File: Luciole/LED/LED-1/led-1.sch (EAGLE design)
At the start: 6 parts, among them Q2 MOSFET-NCHANNELAO3404A

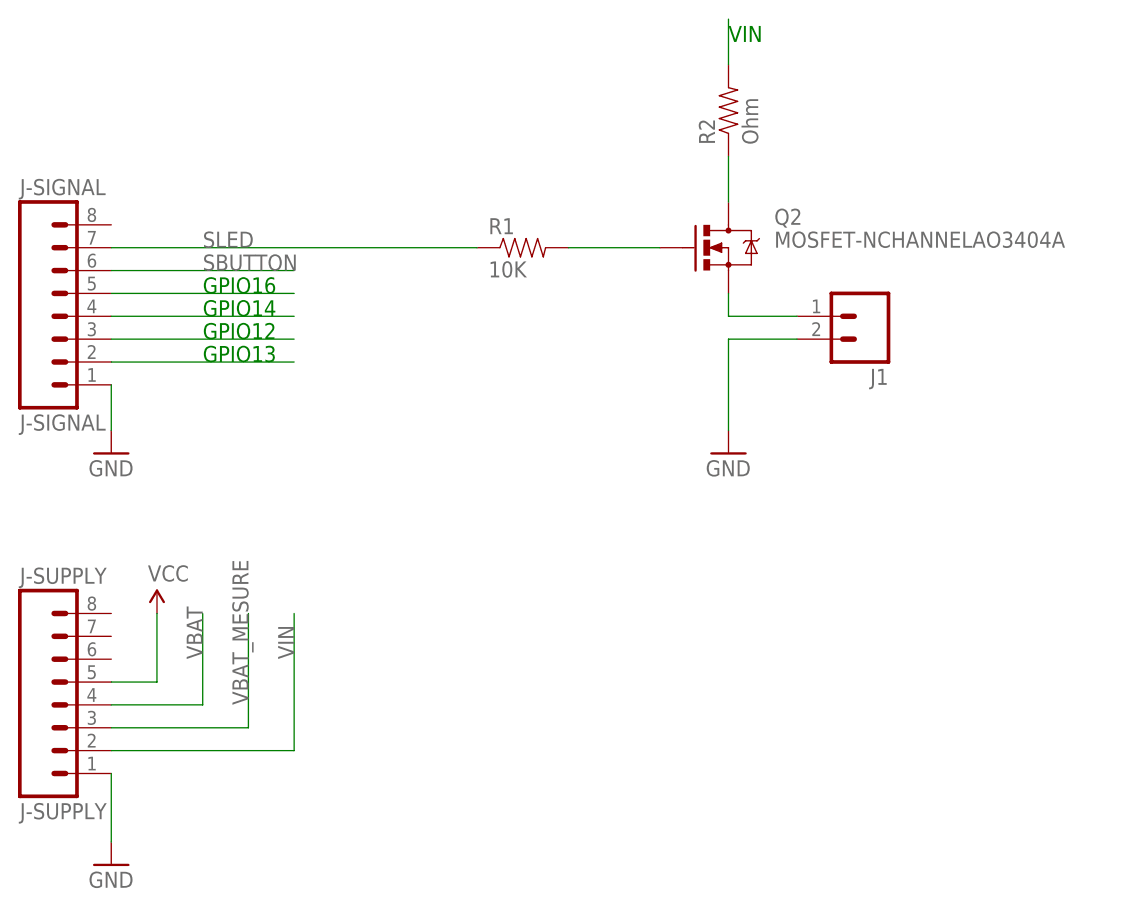
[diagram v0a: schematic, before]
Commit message: V2 de la Baballe
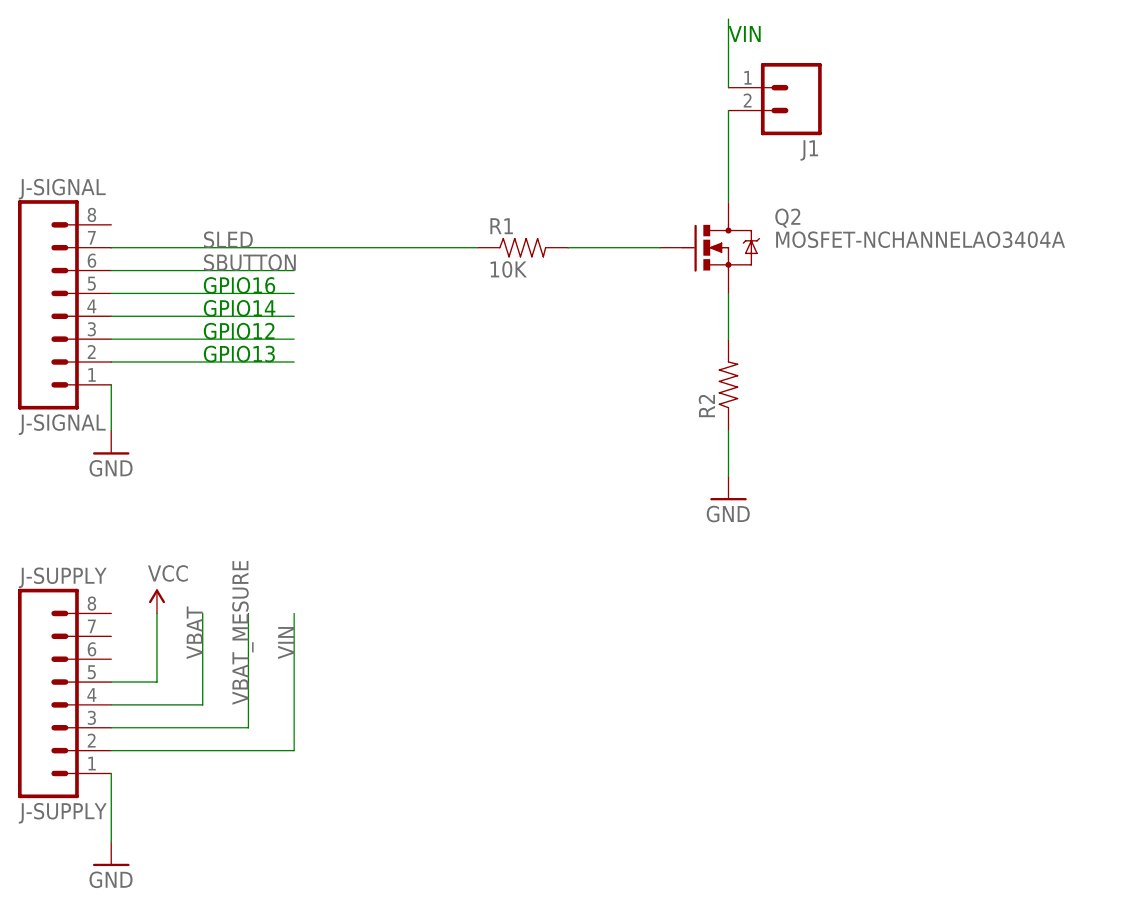
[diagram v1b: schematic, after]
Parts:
- R2: value Ohm -> (none); device SparkFun-Passives:RESISTORPTH-1/4W -> SparkFun-Passives:RESISTORPTH-1/2W
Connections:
- net GND: now also R2.1; no longer J1.2
- net N$1: now also R2.2; no longer J1.1
- net N$3: now also J1.2; no longer R2.1
- net VIN: now also J1.1; no longer R2.2
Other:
- moved on the sheet: J1, R2
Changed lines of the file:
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@@
 <part name="SUPPLY3" library="SparkFun-Aesthetics" deviceset="VCC" device=""/>
 <part name="R1" library="SparkFun-Passives" deviceset="RESISTOR" device="0805-RES" value="10K"/>
-<part name="Q2" library="SparkFun-DiscreteSemi" deviceset="MOSFET-NCHANNEL" device="AO3404A"/>
+<part name="Q2" library="SparkFun-DiscreteSemi" deviceset="MOSFET-NCHANNEL" device="AO3404A" value="MOSFET-NCHANNELAO3404A"/>
 <part name="GND2" library="SparkFun-Aesthetics" deviceset="GND" device=""/>
 <part name="J1" library="SparkFun-Connectors" deviceset="M02" device="JST-PTH-VERT"/>
-<part name="R2" library="SparkFun-Passives" deviceset="RESISTOR" device="PTH-1/4W" value="Ohm"/>
+<part name="R2" library="SparkFun-Passives" deviceset="RESISTOR" device="PTH-1/2W"/>
 </parts>
 <sheets>
@@
 <instance part="R1" gate="G$1" x="-17.78" y="68.58"/>
 <instance part="Q2" gate="G$1" x="5.08" y="68.58"/>
-<instance part="GND2" gate="1" x="5.08" y="45.72"/>
-<instance part="J1" gate="G$1" x="20.32" y="60.96" rot="R180"/>
-<instance part="R2" gate="G$1" x="5.08" y="83.82" rot="R90"/>
+<instance part="GND2" gate="1" x="5.08" y="40.64"/>
+<instance part="J1" gate="G$1" x="12.7" y="86.36" rot="R180"/>
+<instance part="R2" gate="G$1" x="5.08" y="53.34" rot="R90"/>
 </instances>
 <busses>
 </busses>
 <nets>
-<net name="GND" class="0">
+<net name="GND" class="2">
 <segment>
 <pinref part="GND4" gate="1" pin="GND"/>
@@
 </segment>
 <segment>
-<pinref part="J1" gate="G$1" pin="2"/>
-<wire x1="12.7" y1="58.42" x2="5.08" y2="58.42" width="0.1524" layer="91"/>
+<pinref part="R2" gate="G$1" pin="1"/>
 <pinref part="GND2" gate="1" pin="GND"/>
-<wire x1="5.08" y1="58.42" x2="5.08" y2="48.26" width="0.1524" layer="91"/>
+<wire x1="5.08" y1="48.26" x2="5.08" y2="43.18" width="0.1524" layer="91"/>
 </segment>
 </net>
@@
 </segment>
 <segment>
-<pinref part="R2" gate="G$1" pin="2"/>
-<wire x1="5.08" y1="88.9" x2="5.08" y2="93.98" width="0.1524" layer="91"/>
+<wire x1="5.08" y1="86.36" x2="5.08" y2="93.98" width="0.1524" layer="91"/>
+<pinref part="J1" gate="G$1" pin="1"/>
 </segment>
 </net>
@@
 </segment>
 </net>
-<net name="N$1" class="0">
+<net name="N$1" class="2">
 <segment>
 <pinref part="Q2" gate="G$1" pin="S"/>
-<wire x1="5.08" y1="63.5" x2="5.08" y2="60.96" width="0.1524" layer="91"/>
-<wire x1="5.08" y1="60.96" x2="12.7" y2="60.96" width="0.1524" layer="91"/>
-<pinref part="J1" gate="G$1" pin="1"/>
+<pinref part="R2" gate="G$1" pin="2"/>
+<wire x1="5.08" y1="63.5" x2="5.08" y2="58.42" width="0.1524" layer="91"/>
 </segment>
 </net>
-<net name="N$3" class="0">
+<net name="N$3" class="2">
 <segment>
-<pinref part="R2" gate="G$1" pin="1"/>
 <pinref part="Q2" gate="G$1" pin="D"/>
+<pinref part="J1" gate="G$1" pin="2"/>
 <wire x1="5.08" y1="78.74" x2="5.08" y2="73.66" width="0.1524" layer="91"/>
+<wire x1="5.08" y1="78.74" x2="5.08" y2="83.82" width="0.1524" layer="91"/>
 </segment>
 </net>
